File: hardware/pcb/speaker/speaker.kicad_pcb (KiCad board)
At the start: 4 copper layers, 55.4 x 64 mm, 58 parts, among them J1 JST SH BM02B Connector, J2 JST SH BM02B Connector, J3 JST SH BM02B Connector, J4 JST SH BM02B Connector, J5 JST SH BM02B Connector, J6 JST SH BM02B Connector, J7 Conn_01x02, M1 Ultrasonic_Transducer, M10 Ultrasonic_Transducer, M11 Ultrasonic_Transducer, M12 Ultrasonic_Transducer, M13 Ultrasonic_Transducer, M14 Ultrasonic_Transducer, M15 Ultrasonic_Transducer, M16 Ultrasonic_Transducer, M17 Ultrasonic_Transducer, M18 Ultrasonic_Transducer, M19 Ultrasonic_Transducer, M2 Ultrasonic_Transducer, M3 Ultrasonic_Transducer, M4 Ultrasonic_Transducer, M5 Ultrasonic_Transducer, M6 Ultrasonic_Transducer, M7 Ultrasonic_Transducer, M8 Ultrasonic_Transducer, M9 Ultrasonic_Transducer, U1 LTC2631-Z, U2 LM2735XMF

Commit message: add pcb gbr files
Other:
- rule pad_to_mask_clearance: 0.2 -> 0

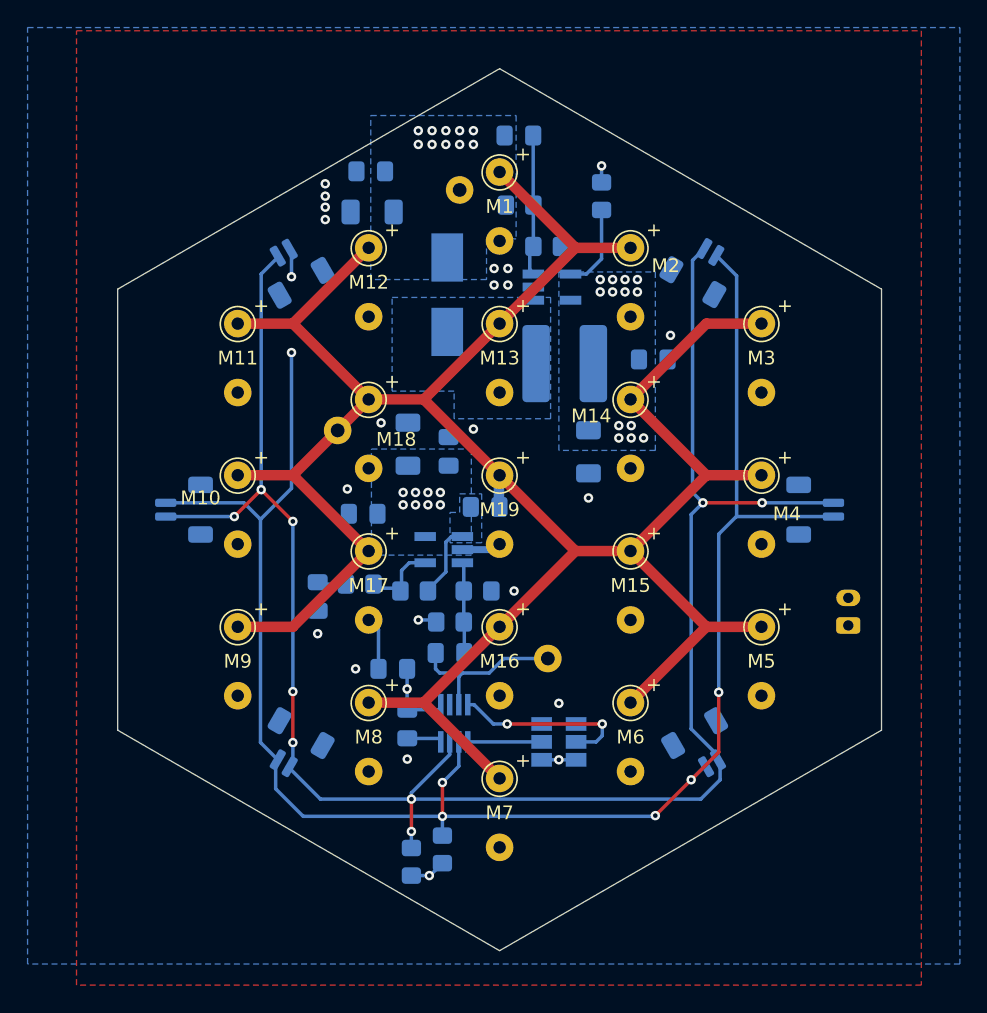
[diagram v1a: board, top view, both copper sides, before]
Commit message: update gerber files
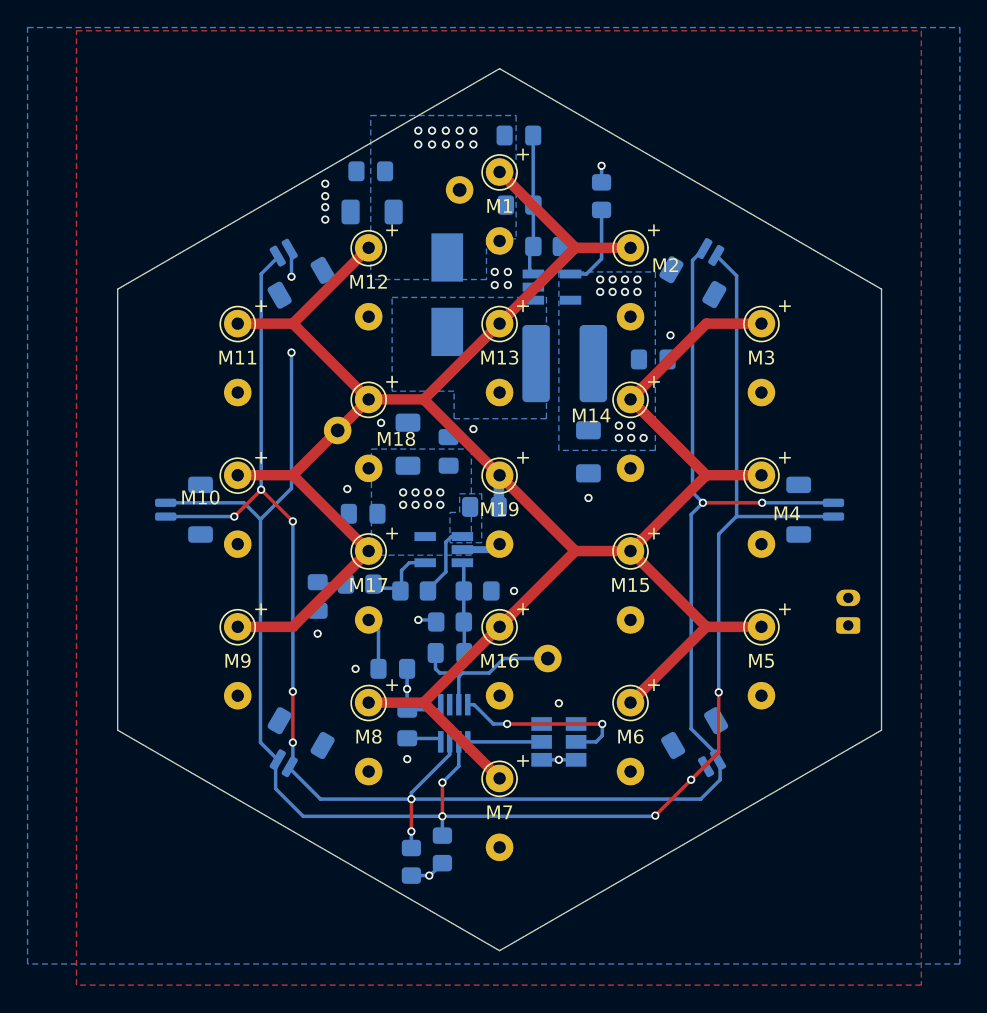
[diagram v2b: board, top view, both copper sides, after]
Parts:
- R1: value 91k -> 180k
- moved C10 0.05 mm to (84.6, 57.0)

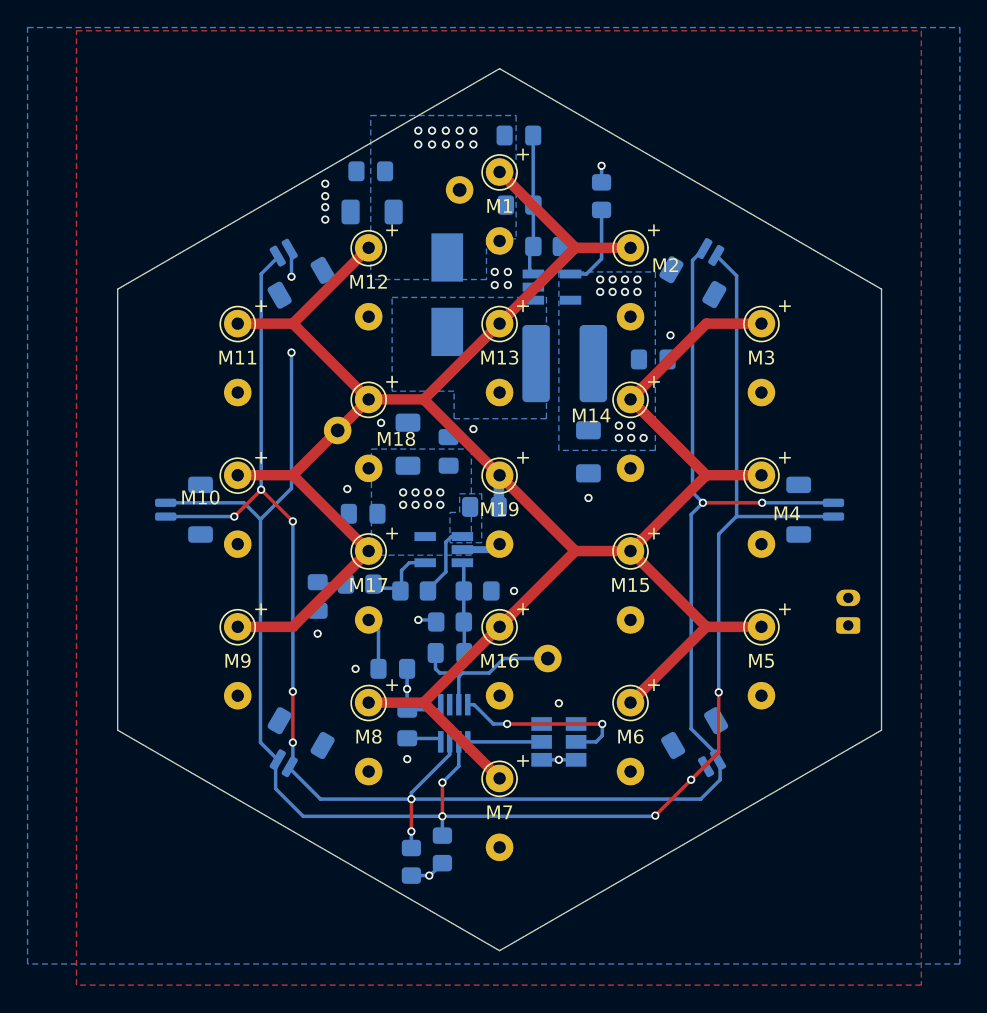
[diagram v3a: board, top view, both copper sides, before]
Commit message: REWORK PCB design
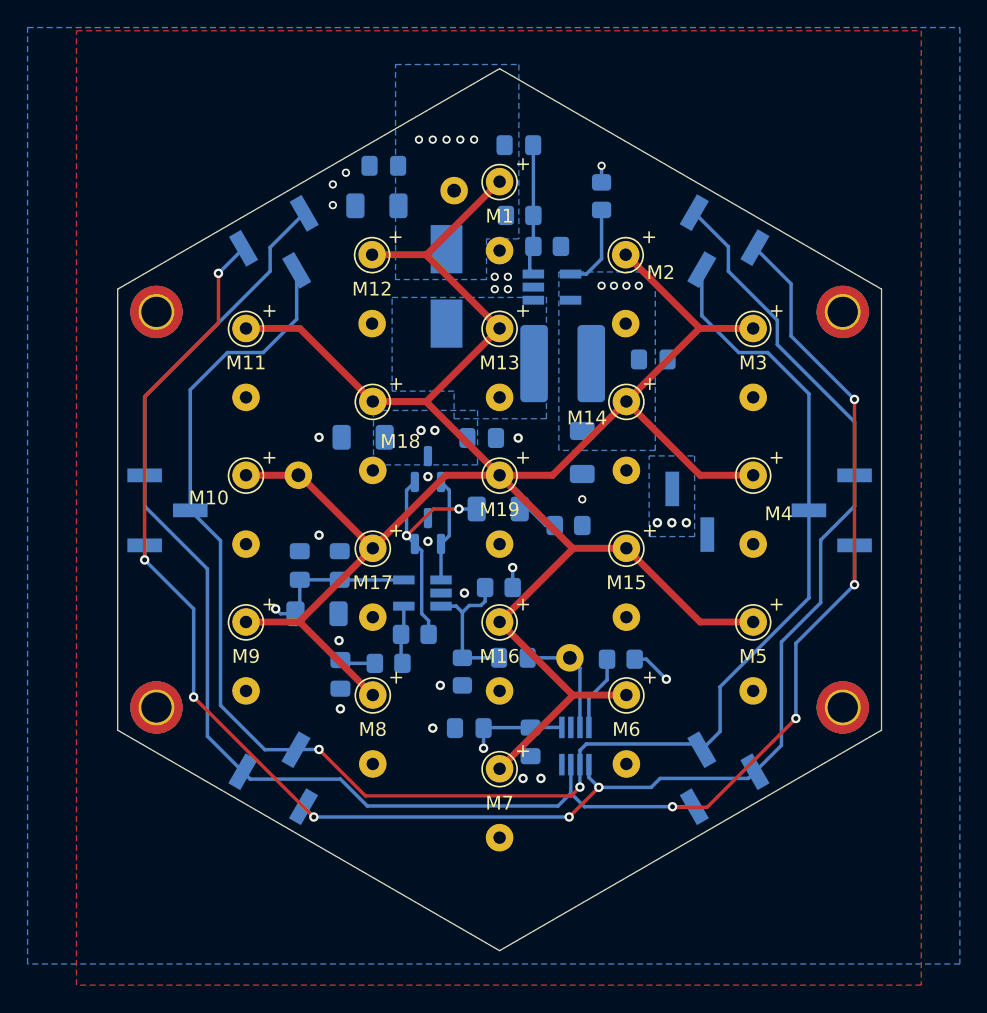
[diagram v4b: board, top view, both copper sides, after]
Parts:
- removed JP2, JP3: Jumper_3_Open, Jumper:SolderJumper-3_P1.3mm_Open_Pad1.0x1.5mm_NumberLabels
- removed R5, R6: 1.5k, Resistor_SMD:R_0805_2012Metric_Pad1.20x1.40mm_HandSolder
- added C14: 10uF, Capacitor_SMD:C_1206_3216Metric_Pad1.33x1.80mm_HandSolder, B.Cu at (75.8, 51.9)
- added C15: 100nF, Capacitor_SMD:C_0805_2012Metric_Pad1.18x1.45mm_HandSolder, B.Cu at (84.4, 52.0)
- added H1: MountingHole_Pad, MountingHole:MountingHole_2.2mm_M2_DIN965_Pad_TopBottom, B.Cu at (60.8, 42.8)
- added H2: MountingHole_Pad, MountingHole:MountingHole_2.2mm_M2_DIN965_Pad_TopBottom, B.Cu at (60.8, 71.5)
- added H3: MountingHole_Pad, MountingHole:MountingHole_2.2mm_M2_DIN965_Pad_TopBottom, B.Cu at (110.6, 71.5)
- added H4: MountingHole_Pad, MountingHole:MountingHole_2.2mm_M2_DIN965_Pad_TopBottom, B.Cu at (110.6, 42.8)
- added Q1: BC847, Package_TO_SOT_SMD:SOT-23, B.Cu at (80.5, 54.2)
- added Q2: BC857, Package_TO_SOT_SMD:SOT-23, B.Cu at (80.5, 58.7)
- added R10: 100k, Resistor_SMD:R_0805_2012Metric_Pad1.20x1.40mm_HandSolder, B.Cu at (90.7, 58.3)
- added R11: 100k, Resistor_SMD:R_0805_2012Metric_Pad1.20x1.40mm_HandSolder, B.Cu at (94.5, 68.0)
- C10: value 100nF -> 1uF; footprint Capacitor_SMD:C_0805_2012Metric_Pad1.18x1.45mm_HandSolder -> Capacitor_SMD:C_1206_3216Metric_Pad1.33x1.80mm_HandSolder
- C8: value 100nF -> 1.5nF
- C9: value 82nF -> 10nF
- J1, J2, J3, J4, J5, J6: value JST SH BM02B Connector -> Conn_01x03; footprint Connector_JST:JST_SH_BM02B-SRSS-TB_1x02-1MP_P1.00mm_Vertical -> custom_footprints:SPI_Conn_SMD
- J7: footprint Connector_JST:JST_PH_B2B-PH-K_1x02_P2.00mm_Vertical -> Connector_PinHeader_2.54mm:PinHeader_1x02_P2.54mm_Vertical_SMD_Pin1Left
- R3: value 10k -> 15k
- R4: value 10k -> 5k
- R8, R9: value 15k -> 100k
- U1: value LTC2631-Z -> LTC2640-Z; footprint custom_footprints:LTC2631-Z -> Package_TO_SOT_SMD:SOT-23-8_Handsoldering
- moved J6 36.1 mm to (101.2, 38.3), turned to -120 degrees
- moved J1 36.1 mm to (70.2, 38.4), turned to -60 degrees
- moved J4 20.3 mm to (101.2, 76.0), turned to 120 degrees
- moved J3 20.2 mm to (70.1, 76.0), turned to 60 degrees
- moved J5 20.0 mm to (109.8, 57.2), turned to 180 degrees
- moved J2 19.8 mm to (61.6, 57.2), turned to 0 degrees
- moved J7 14.2 mm to (99.5, 57.3)
- moved C5 14.0 mm to (72.5, 64.7), turned to 0 degrees
- moved C6 13.6 mm to (71.2, 61.2)
- moved C4 9.04 mm to (88.0, 74.0)
- moved U1 8.66 mm to (91.2, 74.3)
- moved C3 7.02 mm to (83.5, 73.0)
- moved R4 6.12 mm to (77.7, 68.3)
- moved R9 5.95 mm to (83.0, 68.9), turned to -90 degrees
- moved C9 5.89 mm to (74.2, 69.1)
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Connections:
- J1 pad 1: /SDA -> /CS
- J2 pad 1: /SDA -> /CS
- J3 pad 1: /SDA -> /CS
- J4 pad 1: /SDA -> /CS
- J5 pad 1: /SDA -> /CS
- J6 pad 1: /SDA -> /CS
- OP1 pad 1: Net-(C10-Pad1) -> Net-(OP1-Pad1)
- R3 pad 1: Net-(C10-Pad1) -> Net-(OP1-Pad4)
- R3 pad 2: Net-(OP1-Pad4) -> Net-(C10-Pad1)
- U1 pad 1: Net-(JP3-Pad2) -> /CS
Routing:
- net /CS: track 0.00 -> 135.1 mm, vias 0 -> 6
- net /SCL: track 136.0 -> 120.7 mm, vias 7 -> 2
- net Net-(C10-Pad1): track 5.49 -> 17.9 mm, vias 0 -> 2
- net +24V: track 1.39 -> 13.2 mm, vias 19 -> 9
- net GND: track 9.62 -> 0.00 mm, vias 18 -> 20
- net Net-(R11-Pad2): track 13.3 -> 5.50 mm, vias 2 -> 0
- net Net-(OP1-Pad1): track 0.00 -> 7.61 mm
- net /Trancducer Sig: track 182.3 -> 188.4 mm
- net Net-(JP3-Pad2): track 5.36 -> 0.00 mm
- net Net-(C8-Pad2): track 6.71 -> 10.7 mm
- net /Audio Sig: track 12.1 -> 8.41 mm
- net Net-(OP1-Pad4): track 5.80 -> 4.27 mm
- net +5V: track 12.1 -> 11.2 mm, vias 17 -> 10
- net Net-(C7-Pad2): track 10.1 -> 9.42 mm
- net /SDA: track 137.9 -> 138.3 mm, vias 9 -> 4
- removed copper zone on B.Cu, net Net-(C10-Pad1)
